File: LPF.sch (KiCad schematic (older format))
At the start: 142 parts, among them J1 Conn_02x05_Counter_Clockwise, P1 SMA, P2 SMA, P3 SMA, P4 SMA, P5 SMA, P6 SMA

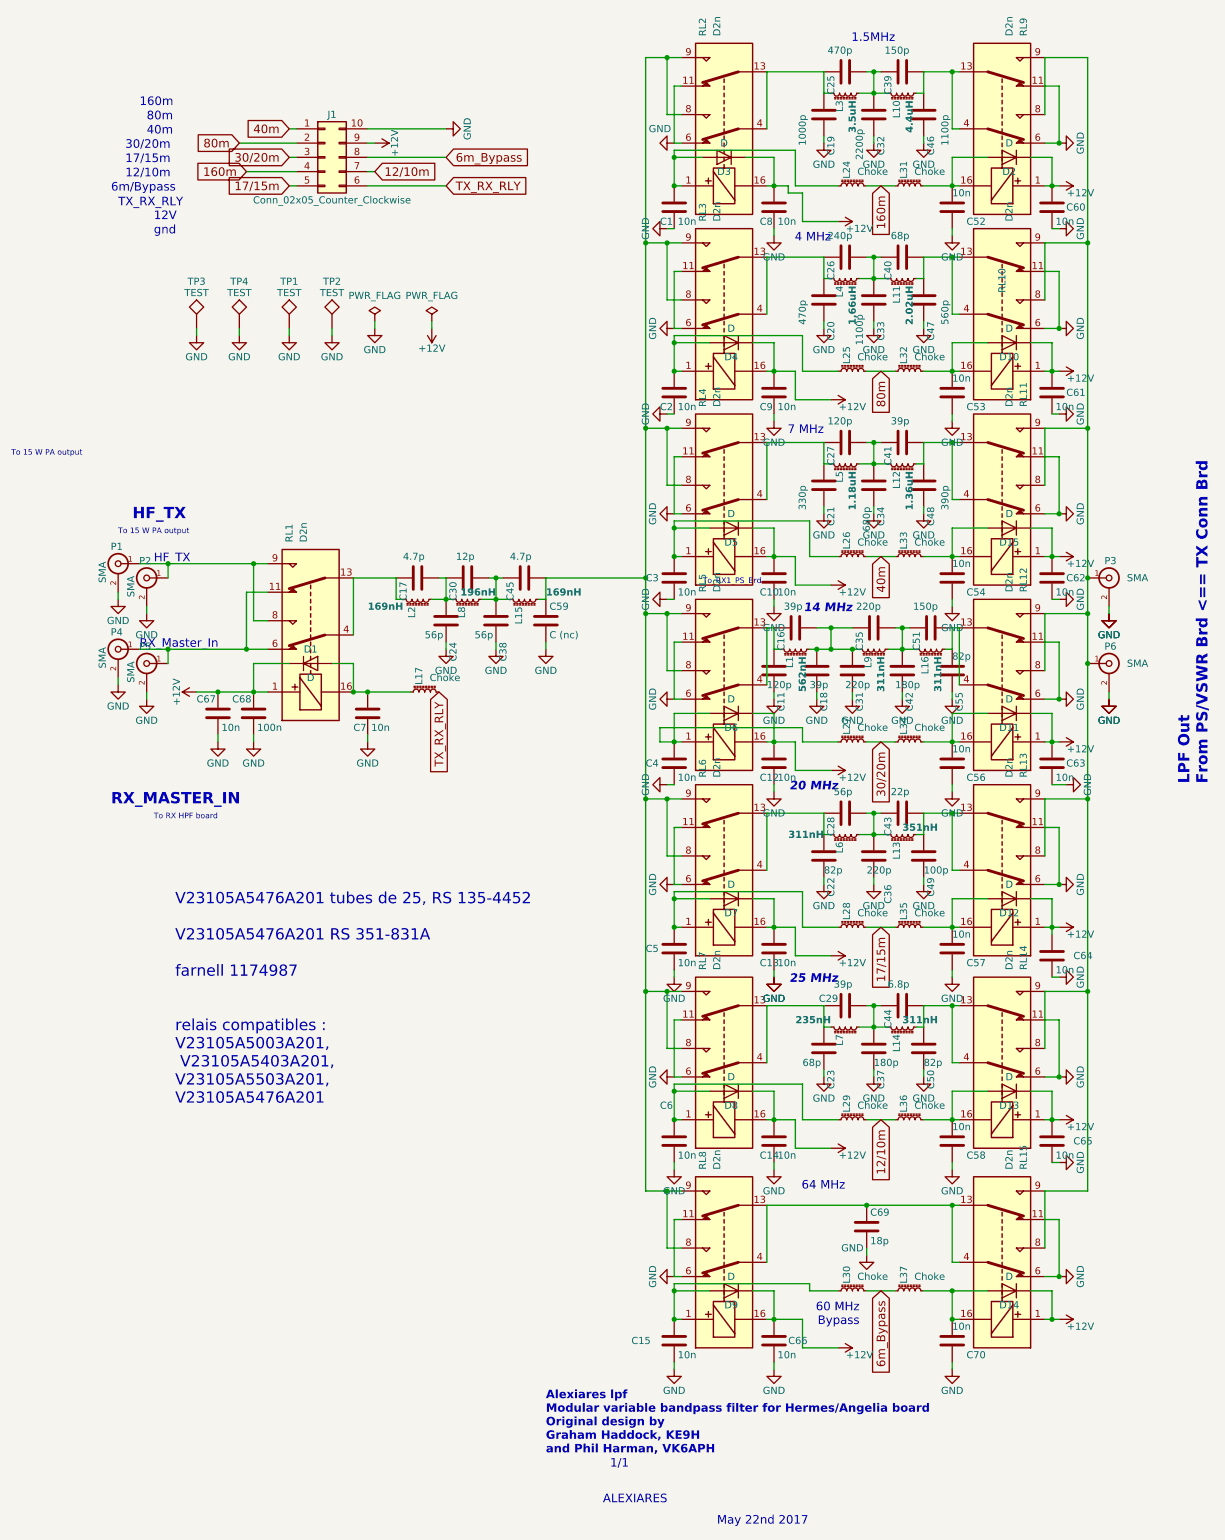
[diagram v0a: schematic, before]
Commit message: V 3.0, 54 MHz lpf now online
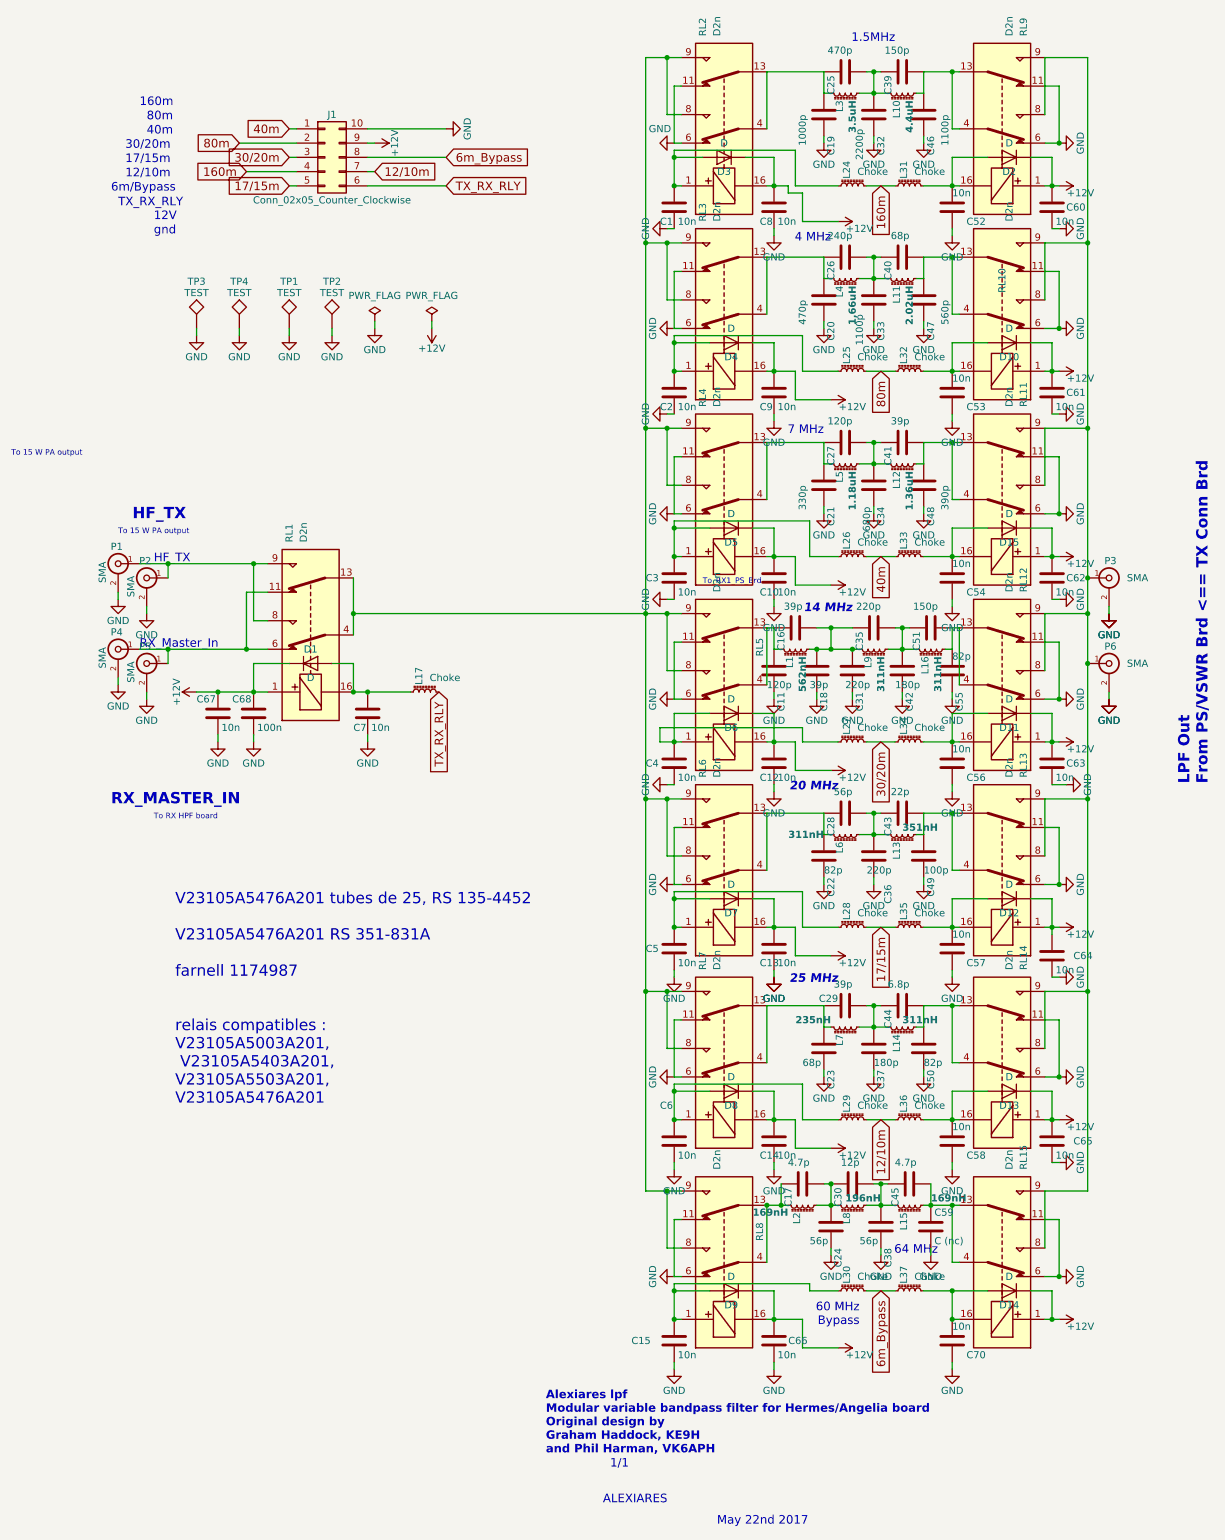
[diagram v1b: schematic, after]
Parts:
- removed C69: 18p, ATC_B:ATC_500_HandSoldering, symbol LPF-rescue:C
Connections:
- net at RL2.8, RL2.9, RL3.8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: now also RL1.13, RL1.4; no longer C45.2, C59.1, L15.2
- net at C17.1, L2.1: now also RL8.13, RL8.4; no longer RL1.13, RL1.4
- net at RL15.13, RL15.4: now also C45.2, C59.1, L15.2; no longer RL8.13, RL8.4
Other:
- moved on the sheet: C17, C24, C30, C38, C45, C59, L15, L2, L8
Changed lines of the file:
@@
 L LPF-rescue:C C45
 U 1 1 592DB317
-P 3450 4400
-F 0 "C45" H 3475 4500 50  0000 L CNN
-F 1 "4.7p" V 3300 4350 50  0000 L CNN
-F 2 "ATC_B:ATC_500_HandSoldering" H 3488 4250 50  0001 C CNN
-F 3 "" H 3450 4400 50  0001 C CNN
-	1    3450 4400
+P 6150 8650
+F 0 "C45" H 6175 8750 50  0000 L CNN
+F 1 "4.7p" V 6000 8600 50  0000 L CNN
+F 2 "ATC_B:ATC_500_HandSoldering" H 6188 8500 50  0001 C CNN
+F 3 "" H 6150 8650 50  0001 C CNN
+	1    6150 8650
 	0    -1   1    0
 $EndComp
@@
 L LPF-rescue:L_Core_Ferrite_Small L15
 U 1 1 592DB318
-P 3450 4550
-F 0 "L15" H 3500 4590 50  0000 L CNN
-F 1 "169nH" V 3400 4150 50  0000 L CNB
-F 2 "T50:T50_V_THT" H 3450 4550 50  0001 C CNN
-F 3 "" H 3450 4550 50  0000 C CNN
-	1    3450 4550
+P 6150 8800
+F 0 "L15" H 6200 8840 50  0000 L CNN
+F 1 "169nH" V 6100 8400 50  0000 L CNB
+F 2 "T50:T50_V_THT" H 6150 8800 50  0001 C CNN
+F 3 "" H 6150 8800 50  0000 C CNN
+	1    6150 8800
 	0    -1   1    0
 $EndComp
@@
 L LPF-rescue:C C38
 U 1 1 592DB319
-P 3250 4700
-F 0 "C38" V 3300 4850 50  0000 L CNN
-F 1 "56p" H 3100 4800 50  0000 L CNN
-F 2 "ATC_B:ATC_500_HandSoldering" H 3288 4550 50  0001 C CNN
-F 3 "" H 3250 4700 50  0001 C CNN
-	1    3250 4700
+P 5950 8950
+F 0 "C38" V 6000 9100 50  0000 L CNN
+F 1 "56p" H 5800 9050 50  0000 L CNN
+F 2 "ATC_B:ATC_500_HandSoldering" H 5988 8800 50  0001 C CNN
+F 3 "" H 5950 8950 50  0001 C CNN
+	1    5950 8950
 	1    0    0    1
 $EndComp
@@
 L LPF-rescue:GND #PWR023
 U 1 1 592DB31A
-P 3250 4900
-F 0 "#PWR023" H 3250 4650 50  0001 C CNN
-F 1 "GND" H 3250 4750 50  0000 C CNN
-F 2 "" H 3250 4900 50  0000 C CNN
-F 3 "" H 3250 4900 50  0000 C CNN
-	1    3250 4900
+P 5950 9150
+F 0 "#PWR023" H 5950 8900 50  0001 C CNN
+F 1 "GND" H 5950 9000 50  0000 C CNN
+F 2 "" H 5950 9150 50  0000 C CNN
+F 3 "" H 5950 9150 50  0000 C CNN
+	1    5950 9150
 	1    0    0    -1
 $EndComp
@@
 L LPF-rescue:C C30
 U 1 1 592DB31B
-P 3050 4400
-F 0 "C30" H 3075 4500 50  0000 L CNN
-F 1 "12p" V 2900 4350 50  0000 L CNN
-F 2 "ATC_B:ATC_500_HandSoldering" H 3088 4250 50  0001 C CNN
-F 3 "" H 3050 4400 50  0001 C CNN
-	1    3050 4400
+P 5750 8650
+F 0 "C30" H 5775 8750 50  0000 L CNN
+F 1 "12p" V 5600 8600 50  0000 L CNN
+F 2 "ATC_B:ATC_500_HandSoldering" H 5788 8500 50  0001 C CNN
+F 3 "" H 5750 8650 50  0001 C CNN
+	1    5750 8650
 	0    -1   1    0
 $EndComp
@@
 L LPF-rescue:L_Core_Ferrite_Small L8
 U 1 1 592DB31C
-P 3050 4550
-F 0 "L8" H 3100 4590 50  0000 L CNN
-F 1 "196nH" V 3000 4350 50  0000 L CNB
-F 2 "T50:T50_V_THT" H 3050 4550 50  0001 C CNN
-F 3 "" H 3050 4550 50  0000 C CNN
-	1    3050 4550
+P 5750 8800
+F 0 "L8" H 5800 8840 50  0000 L CNN
+F 1 "196nH" V 5700 8600 50  0000 L CNB
+F 2 "T50:T50_V_THT" H 5750 8800 50  0001 C CNN
+F 3 "" H 5750 8800 50  0000 C CNN
+	1    5750 8800
 	0    -1   1    0
 $EndComp
@@
 L LPF-rescue:C C24
 U 1 1 592DB31D
-P 2900 4700
-F 0 "C24" V 2950 4850 50  0000 L CNN
-F 1 "56p" H 2750 4800 50  0000 L CNN
-F 2 "ATC_B:ATC_500_HandSoldering" H 2938 4550 50  0001 C CNN
-F 3 "" H 2900 4700 50  0001 C CNN
-	1    2900 4700
+P 5600 8950
+F 0 "C24" V 5650 9100 50  0000 L CNN
+F 1 "56p" H 5450 9050 50  0000 L CNN
+F 2 "ATC_B:ATC_500_HandSoldering" H 5638 8800 50  0001 C CNN
+F 3 "" H 5600 8950 50  0001 C CNN
+	1    5600 8950
 	1    0    0    1
 $EndComp
@@
 L LPF-rescue:GND #PWR024
 U 1 1 592DB31E
-P 2900 4900
-F 0 "#PWR024" H 2900 4650 50  0001 C CNN
-F 1 "GND" H 2900 4750 50  0000 C CNN
-F 2 "" H 2900 4900 50  0000 C CNN
-F 3 "" H 2900 4900 50  0000 C CNN
-	1    2900 4900
+P 5600 9150
+F 0 "#PWR024" H 5600 8900 50  0001 C CNN
+F 1 "GND" H 5600 9000 50  0000 C CNN
+F 2 "" H 5600 9150 50  0000 C CNN
+F 3 "" H 5600 9150 50  0000 C CNN
+	1    5600 9150
 	1    0    0    -1
 $EndComp
@@
 L LPF-rescue:C C17
 U 1 1 592DB343
-P 2700 4400
-F 0 "C17" H 2725 4500 50  0000 L CNN
-F 1 "4.7p" V 2550 4350 50  0000 L CNN
-F 2 "ATC_B:ATC_500_HandSoldering" H 2738 4250 50  0001 C CNN
-F 3 "" H 2700 4400 50  0001 C CNN
-	1    2700 4400
+P 5400 8650
+F 0 "C17" H 5425 8750 50  0000 L CNN
+F 1 "4.7p" V 5250 8600 50  0000 L CNN
+F 2 "ATC_B:ATC_500_HandSoldering" H 5438 8500 50  0001 C CNN
+F 3 "" H 5400 8650 50  0001 C CNN
+	1    5400 8650
 	0    -1   1    0
 $EndComp
@@
 L LPF-rescue:L_Core_Ferrite_Small L2
 U 1 1 592DB344
-P 2700 4550
-F 0 "L2" H 2750 4590 50  0000 L CNN
-F 1 "169nH" V 2750 4650 50  0000 L CNB
-F 2 "T50:T50_V_THT" H 2700 4550 50  0001 C CNN
-F 3 "" H 2700 4550 50  0000 C CNN
-	1    2700 4550
+P 5400 8800
+F 0 "L2" H 5450 8840 50  0000 L CNN
+F 1 "169nH" V 5450 8900 50  0000 L CNB
+F 2 "T50:T50_V_THT" H 5400 8800 50  0001 C CNN
+F 3 "" H 5400 8800 50  0000 C CNN
+	1    5400 8800
 	0    -1   1    0
 $EndComp
@@
 Text Notes 5750 4650 2    60   Italic 12
 14 MHz
-Text Notes 5700 8700 2    60   ~ 0
+Text Notes 6350 9150 2    60   ~ 0
 64 MHz
 Text GLabel 5950 2950 3    60   Input ~ 0
@@
 U 1 1 59F4E319
 P 4850 5350
-F 0 "RL5" H 5700 5500 50  0000 L CNN
+F 0 "RL5" H 5250 5100 50  0000 L CNN
 F 1 "D2n" H 5700 5400 50  0000 L CNN
 F 2 "2_Form_C_Relay:D2n" H 4850 5350 50  0001 C CNN
@@
 L LPF-rescue:C C59
 U 1 1 59FE4103
-P 3600 4700
-F 0 "C59" H 3625 4800 50  0000 L CNN
-F 1 "C (nc)" H 3625 4600 50  0000 L CNN
-F 2 "ATC_B:ATC_500_HandSoldering" H 3638 4550 50  0001 C CNN
-F 3 "" H 3600 4700 50  0001 C CNN
-	1    3600 4700
+P 6300 8950
+F 0 "C59" H 6325 9050 50  0000 L CNN
+F 1 "C (nc)" H 6325 8850 50  0000 L CNN
+F 2 "ATC_B:ATC_500_HandSoldering" H 6338 8800 50  0001 C CNN
+F 3 "" H 6300 8950 50  0001 C CNN
+	1    6300 8950
 	1    0    0    -1
 $EndComp
@@
 L LPF-rescue:GND #PWR078
 U 1 1 59FE4332
-P 3600 4900
-F 0 "#PWR078" H 3600 4650 50  0001 C CNN
-F 1 "GND" H 3600 4750 50  0000 C CNN
-F 2 "" H 3600 4900 50  0000 C CNN
-F 3 "" H 3600 4900 50  0000 C CNN
-	1    3600 4900
+P 6300 9150
+F 0 "#PWR078" H 6300 8900 50  0001 C CNN
+F 1 "GND" H 6300 9000 50  0000 C CNN
+F 2 "" H 6300 9150 50  0000 C CNN
+F 3 "" H 6300 9150 50  0000 C CNN
+	1    6300 9150
 	1    0    0    -1
 $EndComp
@@
 U 1 1 59FDB074
 P 4850 9400
-F 0 "RL8" H 5700 9550 50  0000 L CNN
+F 0 "RL8" H 5200 9150 50  0000 L CNN
 F 1 "D2n" H 5700 9450 50  0000 L CNN
 F 2 "2_Form_C_Relay:D2n" H 4850 9400 50  0001 C CNN
@@
 	0    1    -1   0
 $EndComp
-$Comp
-L LPF-rescue:C C69
-U 1 1 59FDCDC1
-P 5850 8950
-F 0 "C69" H 5875 9050 50  0000 L CNN
-F 1 "18p" H 5875 8850 50  0000 L CNN
-F 2 "ATC_B:ATC_500_HandSoldering" H 5888 8800 50  0001 C CNN
-F 3 "" H 5850 8950 50  0001 C CNN
-	1    5850 8950
-	1    0    0    -1
-$EndComp
-$Comp
-L LPF-rescue:GND #PWR082
-U 1 1 59FDCF49
-P 5850 9150
-F 0 "#PWR082" H 5850 8900 50  0001 C CNN
-F 1 "GND" H 5750 9200 50  0000 C CNN
-F 2 "" H 5850 9150 50  0000 C CNN
-F 3 "" H 5850 9150 50  0000 C CNN
-	1    5850 9150
-	1    0    0    -1
-$EndComp
 Text GLabel 5950 9400 3    60   Input ~ 0
 6m_Bypass
@@
 	6450 4900 6400 4900
 Wire Wire Line
-	3250 4850 3250 4900
+	5950 9100 5950 9150
 Wire Wire Line
-	2900 4850 2900 4900
+	5600 9100 5600 9150
 Wire Wire Line
-	3250 4550 3250 4400
+	5950 8800 5950 8650
 Wire Wire Line
-	3200 4400 3250 4400
-Connection ~ 3250 4400
+	5900 8650 5950 8650
+Connection ~ 5950 8650
 Wire Wire Line
-	3150 4550 3250 4550
-Connection ~ 3250 4550
+	5850 8800 5950 8800
+Connection ~ 5950 8800
 Wire Wire Line
-	2800 4550 2900 4550
+	5500 8800 5600 8800
 Wire Wire Line
-	2900 4550 2900 4400
+	5600 8800 5600 8650
 Wire Wire Line
-	3600 4400 3600 4550
+	6300 8650 6300 8800
 Wire Wire Line
-	3600 4550 3550 4550
+	6300 8800 6250 8800
 Wire Wire Line
 	6250 6050 6450 6050
@@
 Connection ~ 6450 7400
 Wire Wire Line
-	2600 4550 2550 4550
+	5300 8800 5250 8800
 Wire Wire Line
-	2550 4550 2550 4400
-Connection ~ 2900 4550
+	5250 8800 5250 8650
+Connection ~ 5600 8800
 Wire Wire Line
-	2900 4400 2850 4400
+	5600 8650 5550 8650
 Wire Wire Line
 	5500 4750 5600 4750
@@
 Wire Wire Line
 	750  4300 950  4300
-Connection ~ 4300 4400
 Connection ~ 7400 4400
 Wire Wire Line
@@
 	1450 2650 1450 2700
 Wire Wire Line
-	2550 4400 2250 4400
-Wire Wire Line
-	2250 4400 2250 4800
+	2250 4400 2250 4650
 Wire Wire Line
 	1650 4500 1500 4500
@@
 	6500 4750 6500 5150
 Wire Wire Line
-	3600 4400 4300 4400
-Wire Wire Line
 	2900 1250 2350 1250
 Wire Wire Line
@@
 Wire Wire Line
 	2350 5550 2350 5500
-Connection ~ 2350 5200
 Wire Wire Line
-	3600 4850 3600 4900
-Wire Wire Line
-	5150 8800 5850 8800
+	6300 9100 6300 9150
 Wire Wire Line
 	6450 8800 6450 9200
@@
 Wire Wire Line
 	7400 8700 7100 8700
-Connection ~ 6450 8800
 Wire Wire Line
 	4550 8900 4500 8900
@@
 Wire Wire Line
 	5150 8800 5150 9200
-Connection ~ 5850 8800
-Wire Wire Line
-	5850 9100 5850 9150
 Wire Wire Line
 	4500 9900 4500 9950
@@
 	6100 4900 6200 4900
 Wire Wire Line
-	3250 4400 3300 4400
+	5950 8650 6000 8650
 Wire Wire Line
-	3250 4550 3350 4550
+	5950 8800 6050 8800
 Wire Wire Line
 	7150 6850 7200 6850
@@
 	6450 7400 6500 7400
 Wire Wire Line
-	2900 4550 2950 4550
+	5600 8800 5650 8800
 Wire Wire Line
 	4500 5550 4550 5550
@@
 	4300 2050 4300 3350
 Wire Wire Line
-	4300 3350 4300 4400
-Wire Wire Line
 	4300 4650 4300 5950
 Wire Wire Line
@@
 	4300 7300 4300 8700
 Wire Wire Line
-	4300 4400 4300 4650
-Wire Wire Line
 	7400 4400 7400 4650
 Wire Wire Line
@@
 	4450 8700 4550 8700
 Wire Wire Line
-	5850 8800 6450 8800
-Wire Wire Line
 	5200 1650 5300 1650
 Wire Wire Line
@@
 Wire Wire Line
 	5850 8200 6050 8200
+Connection ~ 5600 8650
+Connection ~ 6300 8800
+Wire Wire Line
+	4300 3350 4300 4650
+Connection ~ 2350 5200
+Wire Wire Line
+	6300 8800 6450 8800
+Connection ~ 6450 8800
+Wire Wire Line
+	5250 8800 5150 8800
+Connection ~ 5250 8800
+Connection ~ 5150 8800
+Wire Wire Line
+	4300 4650 2250 4650
+Connection ~ 2250 4650
+Wire Wire Line
+	2250 4650 2250 4800
 $EndSCHEMATC

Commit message: version 3 provisoire
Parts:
- RL1, RL10, RL11, RL12, RL13, RL14, RL15, RL2, RL3, RL4, RL5, RL6, RL7, RL8, RL9: symbol d2n:D2n -> LPF-rescue:D2n-d2n
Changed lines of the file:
@@
 EESchema Schematic File Version 4
-LIBS:LPF-cache
-EELAYER 26 0
+EELAYER 30 0
 EELAYER END
 $Descr A4 8268 11693 portrait
@@
 P 5950 9150
 F 0 "#PWR023" H 5950 8900 50  0001 C CNN
-F 1 "GND" H 5950 9000 50  0000 C CNN
+F 1 "GND" H 5900 9100 50  0000 C CNN
 F 2 "" H 5950 9150 50  0000 C CNN
 F 3 "" H 5950 9150 50  0000 C CNN
@@
 P 5600 9150
 F 0 "#PWR024" H 5600 8900 50  0001 C CNN
-F 1 "GND" H 5600 9000 50  0000 C CNN
+F 1 "GND" H 5500 9100 50  0000 C CNN
 F 2 "" H 5600 9150 50  0000 C CNN
 F 3 "" H 5600 9150 50  0000 C CNN
@@
 HF_TX
 $Comp
-L d2n:D2n RL12
+L LPF-rescue:D2n-d2n RL12
 U 1 1 59F4CD62
 P 6800 5350
@@
 $EndComp
 $Comp
-L d2n:D2n RL2
+L LPF-rescue:D2n-d2n RL2
 U 1 1 59F4E038
 P 4850 1450
@@
 $EndComp
 $Comp
-L d2n:D2n RL3
+L LPF-rescue:D2n-d2n RL3
 U 1 1 59F4E18A
 P 4850 2750
@@
 $EndComp
 $Comp
-L d2n:D2n RL4
+L LPF-rescue:D2n-d2n RL4
 U 1 1 59F4E24B
 P 4850 4050
@@
 $EndComp
 $Comp
-L d2n:D2n RL5
+L LPF-rescue:D2n-d2n RL5
 U 1 1 59F4E319
 P 4850 5350
@@
 $EndComp
 $Comp
-L d2n:D2n RL1
+L LPF-rescue:D2n-d2n RL1
 U 1 1 59F4E3D0
 P 1950 5000
@@
 $EndComp
 $Comp
-L d2n:D2n RL6
+L LPF-rescue:D2n-d2n RL6
 U 1 1 59F4E6AC
 P 4850 6650
@@
 $EndComp
 $Comp
-L d2n:D2n RL7
+L LPF-rescue:D2n-d2n RL7
 U 1 1 59F4E779
 P 4850 8000
@@
 $EndComp
 $Comp
-L d2n:D2n RL10
+L LPF-rescue:D2n-d2n RL10
 U 1 1 59F51169
 P 6800 2750
@@
 $EndComp
 $Comp
-L d2n:D2n RL11
+L LPF-rescue:D2n-d2n RL11
 U 1 1 59F5159A
 P 6800 4050
@@
 $EndComp
 $Comp
-L d2n:D2n RL13
+L LPF-rescue:D2n-d2n RL13
 U 1 1 59F518D7
 P 6800 6650
@@
 $EndComp
 $Comp
-L d2n:D2n RL14
+L LPF-rescue:D2n-d2n RL14
 U 1 1 59F5236E
 P 6800 8000
@@
 P 6300 9150
 F 0 "#PWR078" H 6300 8900 50  0001 C CNN
-F 1 "GND" H 6300 9000 50  0000 C CNN
+F 1 "GND" H 6250 9100 50  0000 C CNN
 F 2 "" H 6300 9150 50  0000 C CNN
 F 3 "" H 6300 9150 50  0000 C CNN
@@
 60 MHz\nBypass\n
 $Comp
-L d2n:D2n RL8
+L LPF-rescue:D2n-d2n RL8
 U 1 1 59FDB074
 P 4850 9400
@@
 $EndComp
 $Comp
-L d2n:D2n RL15
+L LPF-rescue:D2n-d2n RL15
 U 1 1 59FDB07A
 P 6800 9400
@@
 $EndComp
 $Comp
-L d2n:D2n RL9
+L LPF-rescue:D2n-d2n RL9
 U 1 1 59F50E3A
 P 6800 1450
